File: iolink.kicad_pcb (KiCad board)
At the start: 2 copper layers, 47 parts, among them IC1 LTC2874IFE#PBF, IC2 AZ1117CH2-5.0TRG1, IC3 M78AR05-0.5, IC4 CH224K, J1 Screw_Terminal_01x04, J2 USB_C_Receptacle_USB2.0, J3 Screw_Terminal_01x05, J4 Screw_Terminal_01x04, J5 Screw_Terminal_01x04, J6 Screw_Terminal_01x04, J7 Screw_Terminal_01x04, Q1 NDS9936, Q2 NDS9936, SW1 SW_Push, U1 STM32F091CCTx, U2 MCP2562-H-SN, Y1 8Mhz

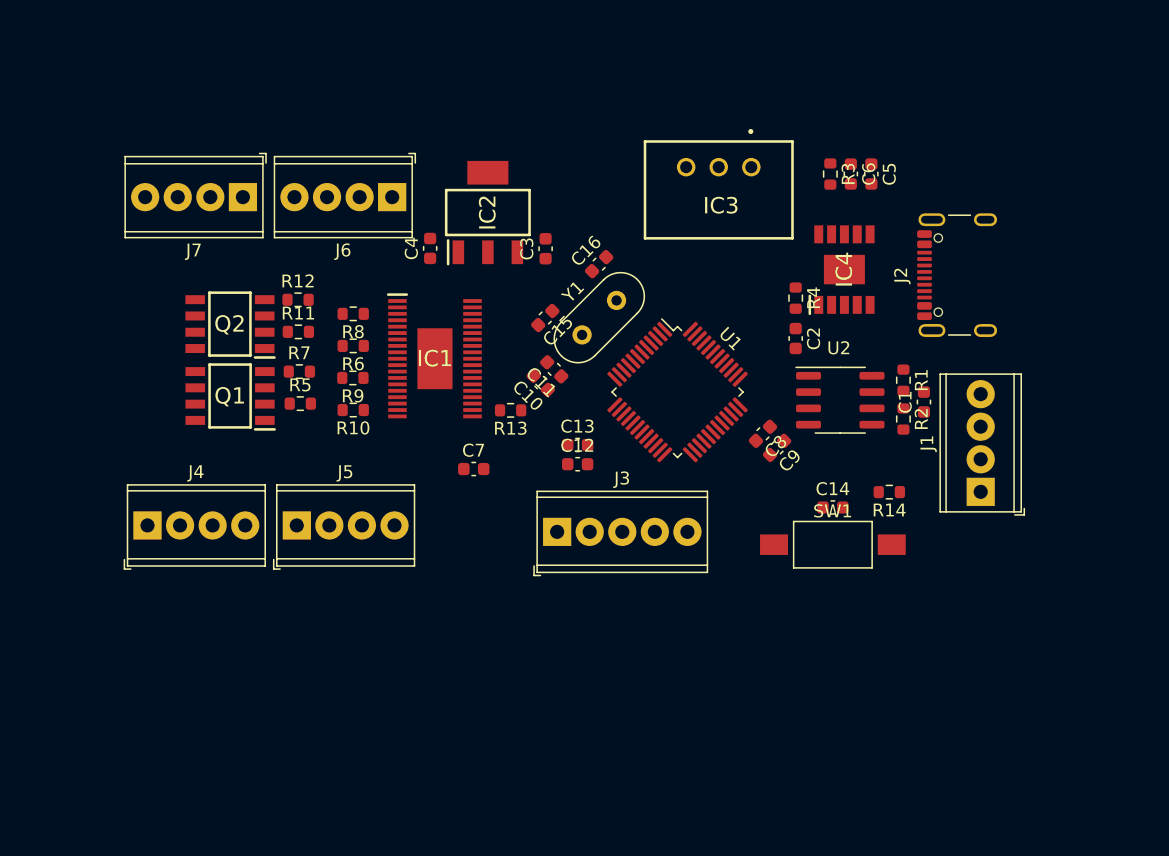
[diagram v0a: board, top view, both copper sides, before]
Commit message: temp
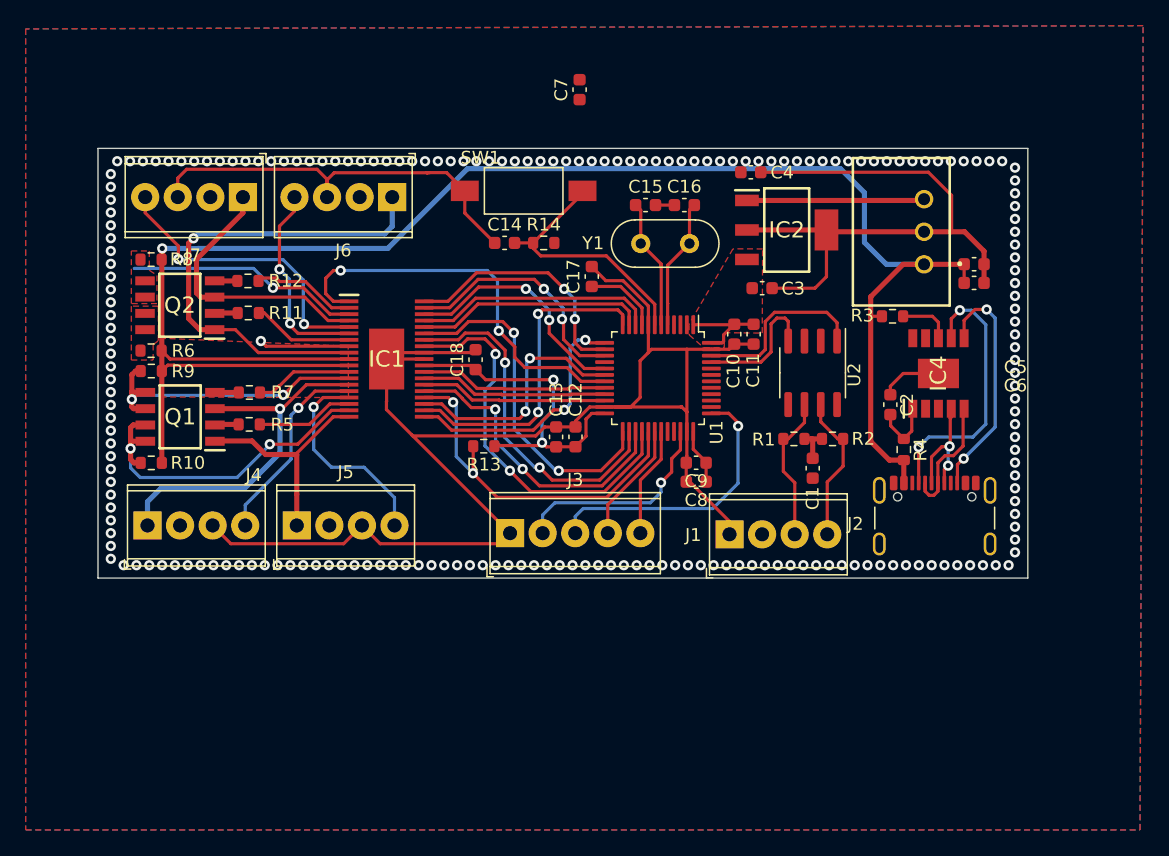
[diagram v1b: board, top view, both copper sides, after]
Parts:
- added C17: 0.1uF, Capacitor_SMD:C_0603_1608Metric, F.Cu at (89.5, 80.0)
- added C18: 4.7uF, Capacitor_SMD:C_0603_1608Metric, F.Cu at (80.4, 86.5)
- moved SW1 36.6 mm to (84.2, 73.3)
- moved R14 33.2 mm to (85.8, 77.4), turned to 0 degrees
- moved C14 32.9 mm to (82.7, 77.4)
- moved C7 30.7 mm to (88.5, 65.4), turned to 90 degrees
- moved C4 25.7 mm to (101.9, 71.9), turned to 0 degrees
- moved IC2 23.3 mm to (104.7, 76.4), turned to 0 degrees
- moved J2 20.1 mm to (116.2, 99.8), turned to 0 degrees
- moved J1 19.9 mm to (100.2, 100.1), turned to 0 degrees
- moved IC3 19.3 mm to (117.4, 76.5), turned to 90 degrees
- moved C3 17.2 mm to (102.8, 80.9), turned to 0 degrees
- moved R8 16.3 mm to (55.1, 78.7), turned to 0 degrees
- moved R10 16.3 mm to (55.2, 94.5), turned to 0 degrees
- moved C11 15.8 mm to (102.1, 84.5), turned to -90 degrees
- moved R6 15.8 mm to (55.1, 85.8), turned to 0 degrees
- moved R9 15.7 mm to (55.2, 87.4), turned to 0 degrees
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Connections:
- J1 pad 3: /CAN_H -> /CAN_L
- J1 pad 4: /CAN_L -> /CAN_H
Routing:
- net GND: track 0.00 -> 203.3 mm, vias 0 -> 202
- net VBUS: track 0.00 -> 140.7 mm, vias 0 -> 1
- net +3V3: track 0.00 -> 43.8 mm, vias 0 -> 2
- net Net-(IC1-L+3): track 0.00 -> 38.6 mm, vias 0 -> 1
- net /USART6_EN: track 0.00 -> 31.6 mm, vias 0 -> 2
- net /SPI2_MOSI: track 0.00 -> 30.7 mm, vias 0 -> 2
- net Net-(IC1-L+2): track 0.00 -> 28.6 mm, vias 0 -> 1
- net /IRQ: track 0.00 -> 28.4 mm, vias 0 -> 2
- net /SPI2_SCK: track 0.00 -> 27.4 mm, vias 0 -> 2
- net /SPI2_NSS: track 0.00 -> 27.1 mm, vias 0 -> 2
- net Net-(IC1-SENSE-1): track 0.00 -> 26.8 mm, vias 0 -> 2
- net /USART2_TX: track 0.00 -> 25.3 mm, vias 0 -> 2
- net /SPI2_MISO: track 0.00 -> 23.7 mm, vias 0 -> 2
- net Net-(IC1-CQ4): track 0.00 -> 23.4 mm, vias 0 -> 2
- net Net-(IC1-SENSE-2): track 0.00 -> 23.1 mm, vias 0 -> 2
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- added copper zone on F.Cu, net +3V3
- added copper zone on B.Cu, net GND
- added copper zone on F.Cu, net GND
- added copper zone on F.Cu, net Net-(IC1-SENSE-3)
- added copper zone on F.Cu, net Net-(IC1-SENSE-4)
- added copper zone on F.Cu, net VBUS
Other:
- board outline added: 72.5 x 33.5 mm

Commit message: complete
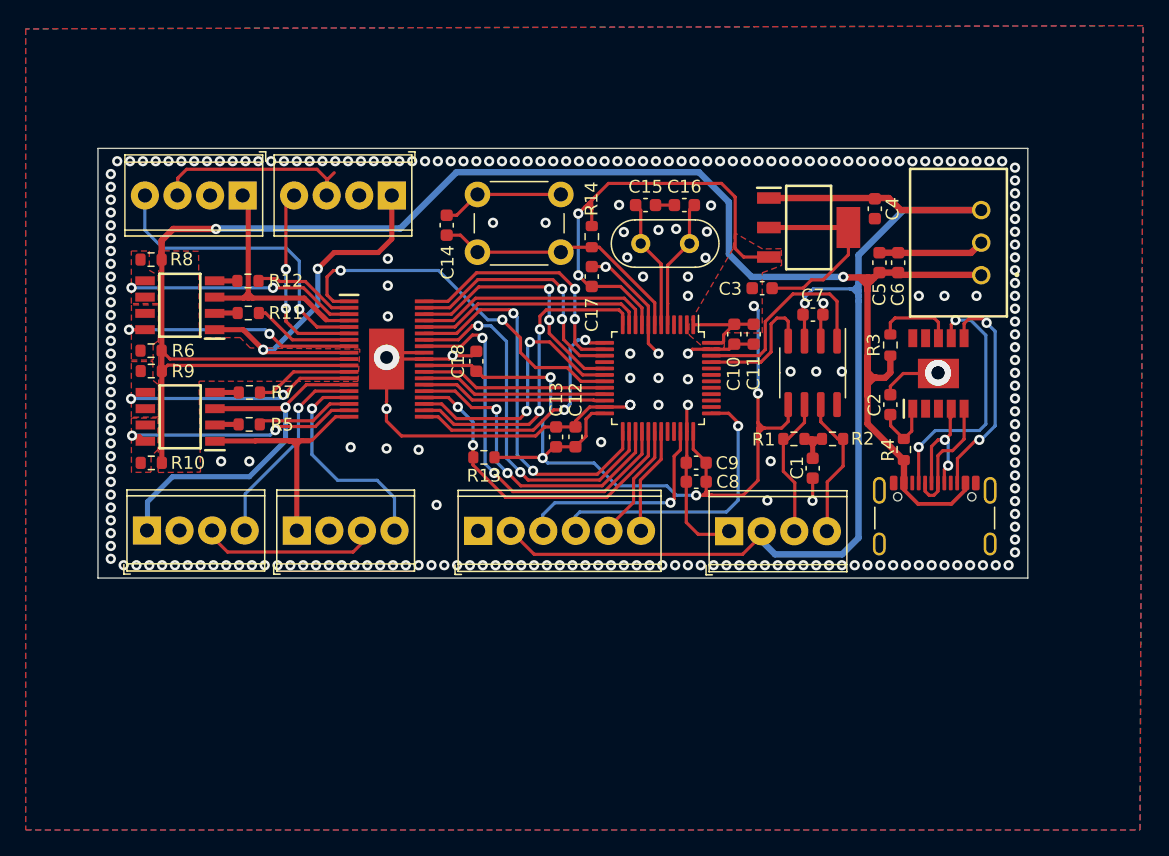
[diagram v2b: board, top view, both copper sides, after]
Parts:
- removed J3: Screw_Terminal_01x05, TerminalBlock_Phoenix:TerminalBlock_Phoenix_MPT-0,5-5-2.54_1x05_P2.54mm_Horizontal
- added J8: Screw_Terminal_01x06, TerminalBlock_Phoenix:TerminalBlock_Phoenix_MPT-0,5-6-2.54_1x06_P2.54mm_Horizontal, F.Cu at (80.6, 99.8)
- C14: value C -> 0.1uf
- C7: value 4.7uF -> 0.1uF
- SW1: footprint Button_Switch_SMD:SW_SPST_FSMSM -> Button_Switch_THT:SW_PUSH_6mm
- moved C7 25.3 mm to (106.7, 83.0), turned to 0 degrees
- moved C4 10.1 mm to (111.6, 74.7), turned to -90 degrees
- moved C5 7.38 mm to (111.9, 78.9), turned to 90 degrees
- moved C6 6.13 mm to (113.4, 78.9), turned to 90 degrees
- moved C14 4.72 mm to (78.2, 76.0), turned to -90 degrees
- moved IC3 4.54 mm to (121.9, 77.3)
- moved R14 3.78 mm to (89.5, 76.9), turned to 90 degrees
- moved SW1 3.61 mm to (80.6, 73.6)
- moved R3 2.25 mm to (112.8, 85.3), turned to 90 degrees
- moved IC2 1.72 mm to (106.4, 76.2)
- moved R13 0.87 mm to (81.1, 94.1)
- moved J5 0.40 mm to (66.5, 99.8)
- moved J4 0.39 mm to (54.8, 99.8)
- moved J1 0.24 mm to (100.2, 99.8)
- moved C18 0.14 mm to (80.5, 86.6)
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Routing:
- net +5V: track 13.9 -> 90.2 mm, vias 0 -> 1
- net +3V3: track 43.8 -> 115.9 mm, vias 2 -> 7
- net GND: track 203.3 -> 141.3 mm, vias 202 -> 251
- net VBUS: track 140.7 -> 153.3 mm, vias 1 -> 2
- net Net-(IC1-SENSE-3): track 7.05 -> 18.9 mm, vias 1 -> 2
- net Net-(IC1-L+3): track 38.6 -> 30.3 mm, vias 1 -> 2
- net Net-(IC1-SENSE-1): track 26.8 -> 19.0 mm
- net Net-(IC1-SENSE-2): track 23.1 -> 17.7 mm
- net /SPI2_NSS: track 27.1 -> 30.0 mm
- net Net-(IC1-L+1): track 20.8 -> 23.1 mm
- net /CAN_TX: track 13.6 -> 15.7 mm
- net /USART6_EN: track 31.6 -> 29.4 mm
- net Net-(IC4-VBUS): track 4.19 -> 6.20 mm
- net /USART2_EN: track 19.3 -> 21.1 mm
- net /SPI2_SCK: track 27.4 -> 29.2 mm
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- added copper zone on F.Cu, net Net-(IC1-SENSE-1)
- added copper zone on F.Cu, net Net-(IC1-SENSE-2)
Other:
- board text added: "1uF"
